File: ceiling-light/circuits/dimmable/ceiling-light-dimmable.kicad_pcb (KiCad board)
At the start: 2 copper layers, 100 x 100 mm, 21 parts, among them J1 Screw_Terminal_01x03, J2 Screw_Terminal_01x02, Q1 BT136-500, SW1 SW_Push, U1 LTV-817, U2 HLK-PM05, U3 MOC3021M, U4 WeMos_mini

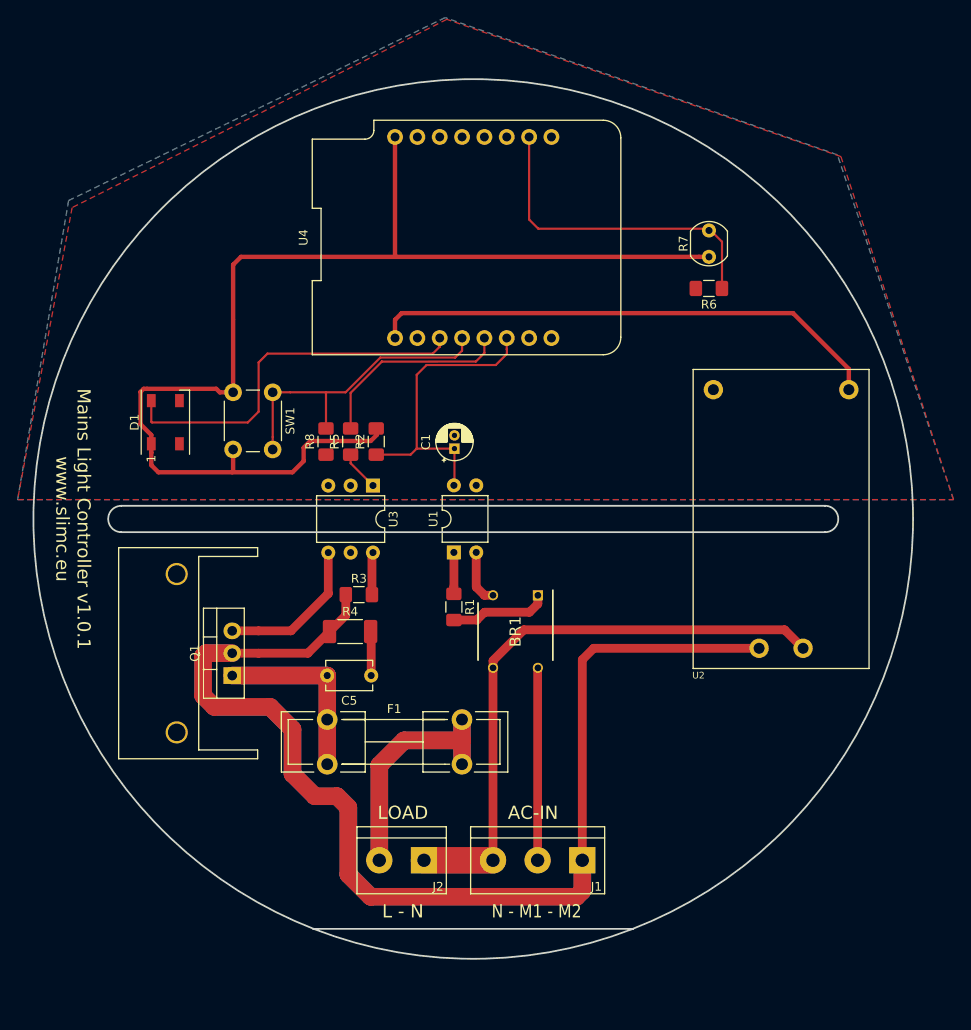
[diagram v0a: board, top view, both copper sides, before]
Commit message: work on dimmable circuit and git submodules
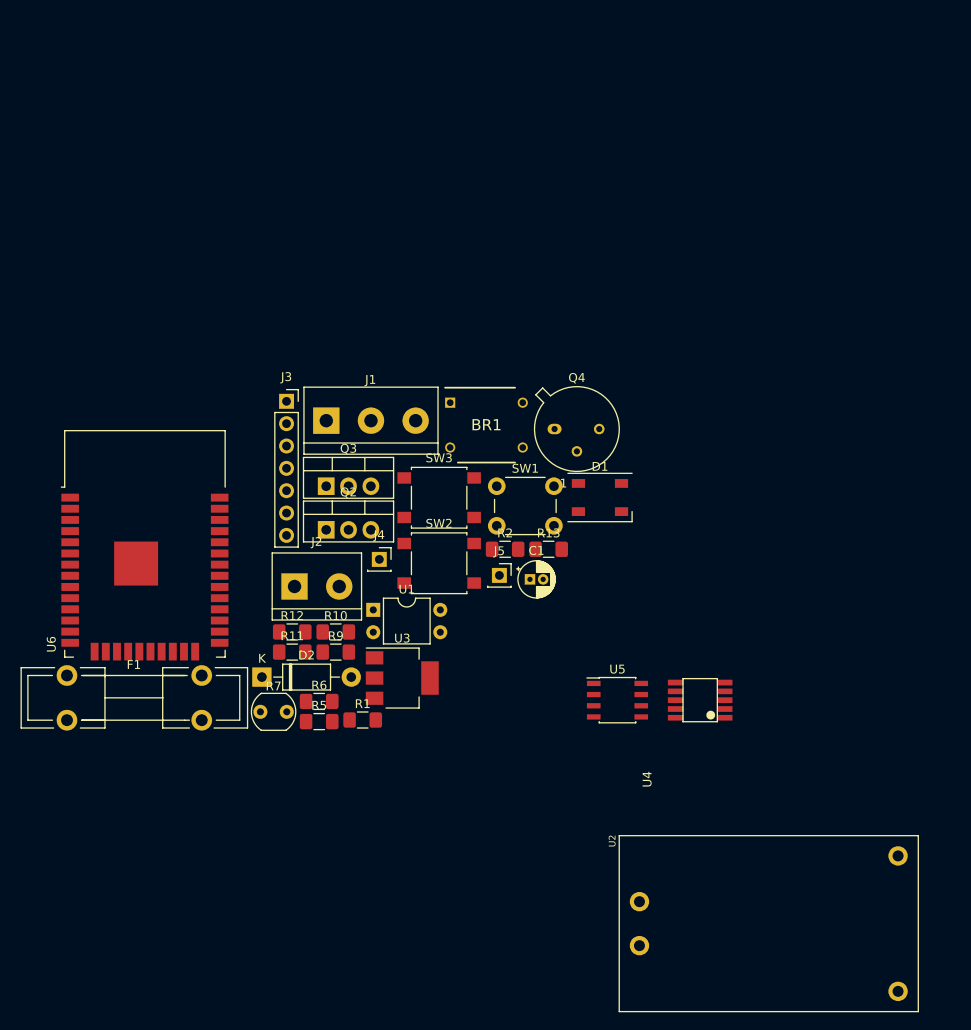
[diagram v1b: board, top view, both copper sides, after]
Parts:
- removed C5: 100NF, Capacitor_THT:C_Disc_D5.1mm_W3.2mm_P5.00mm
- removed Q1: BT136-500, slimc:TO-220-3_Vertical_Triode_Heatsink
- removed R3, R8: 10K, Resistor_SMD:R_1206_3216Metric_Pad1.42x1.75mm_HandSolder
- removed R4: 100R, Resistor_SMD:R_2010_5025Metric_Pad1.52x2.65mm_HandSolder
- added D2: 1N4007, Diode_THT:D_DO-41_SOD81_P10.16mm_Horizontal, F.Cu at (41.0, 83.0)
- added J3: Conn_01x07, Connector_PinSocket_2.54mm:PinSocket_1x07_P2.54mm_Vertical, F.Cu at (43.8, 51.6)
- added J4: Conn_01x01, Connector_PinSocket_2.54mm:PinSocket_1x01_P2.54mm_Vertical, F.Cu at (54.3, 69.6)
- added J5: Conn_01x01, Connector_PinSocket_2.54mm:PinSocket_1x01_P2.54mm_Vertical, F.Cu at (68.0, 71.4)
- added Q2: IRF840, Package_TO_SOT_THT:TO-220-3_Vertical, F.Cu at (48.3, 66.2)
- added Q3: IRF840, Package_TO_SOT_THT:TO-220-3_Vertical, F.Cu at (48.3, 61.3)
- added Q4: KSP44, Package_TO_SOT_THT:TO-39-3, F.Cu at (74.2, 54.8)
- added R10: 2M, Resistor_SMD:R_1206_3216Metric_Pad1.42x1.75mm_HandSolder, F.Cu at (49.4, 77.8)
- added R11: 1K, Resistor_SMD:R_1206_3216Metric_Pad1.42x1.75mm_HandSolder, F.Cu at (44.4, 80.1)
- added R12: 2M, Resistor_SMD:R_1206_3216Metric_Pad1.42x1.75mm_HandSolder, F.Cu at (44.4, 77.8)
- added R13: 2M, Resistor_SMD:R_1206_3216Metric_Pad1.42x1.75mm_HandSolder, F.Cu at (73.6, 68.4)
- added R9: 33K, Resistor_SMD:R_1206_3216Metric_Pad1.42x1.75mm_HandSolder, F.Cu at (49.4, 80.1)
- added SW2: SW_Push, Button_Switch_SMD:SW_SPST_B3S-1000, F.Cu at (61.1, 70.0)
- added SW3: SW_Push, Button_Switch_SMD:SW_SPST_B3S-1000, F.Cu at (61.1, 62.6)
- added U5: TMP36xS, Package_SO:SOIC-8_3.9x4.9mm_P1.27mm, F.Cu at (81.4, 85.6)
- added U6: ESP32-WROOM-32D, RF_Module:ESP32-WROOM-32, F.Cu at (27.7, 70.8)
- R5: value 33R -> 330K
- R6: value 10K -> 6K8
- U3: value MOC3021M -> AMS1117-3.3; footprint Package_DIP:DIP-6_W7.62mm -> Package_TO_SOT_SMD:SOT-223-3_TabPin2
- U4: value WeMos_mini -> FL51xxMX; footprint wemos-d1-mini:wemos-d1-mini-connectors-only -> slimc:FL51xxMX
- moved R7 72.6 mm to (40.8, 86.9), turned to 0 degrees
- moved R6 64.6 mm to (47.5, 85.7), turned to 0 degrees
- moved U4 58.6 mm to (90.8, 85.6), turned to 90 degrees
- moved J1 57.8 mm to (48.3, 53.8), turned to 0 degrees
- moved D1 50.1 mm to (79.4, 62.6), turned to 0 degrees
- moved U2 46.0 mm to (98.6, 111.0), turned to 0 degrees
- moved J2 34.4 mm to (44.7, 72.7), turned to 0 degrees
- moved R5 32.0 mm to (47.5, 88.0), turned to 0 degrees
- moved F1 30.0 mm to (18.8, 82.8)
- moved SW1 27.6 mm to (67.7, 61.3), turned to 0 degrees
- moved BR1 23.7 mm to (66.5, 54.3), turned to 0 degrees
- moved U3 22.1 mm to (56.9, 83.1), turned to 0 degrees
- moved R2 19.1 mm to (68.6, 68.4), turned to 0 degrees
- moved C1 17.2 mm to (71.4, 71.9), turned to 0 degrees
- moved R1 16.5 mm to (52.4, 87.9), turned to 0 degrees
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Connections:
- net M1_IN renamed /M1_IN
- net M2_IN renamed /M2_IN
- net N_MAIN renamed /N_MAIN
- C1 pad 1: D1 -> /MAINS_SENSE
- D1 pad 4: D4 -> /STATUS_LED
- F1 pad 1: L_OUT -> /L_OUT
- R2 pad 1: D1 -> /MAINS_SENSE
- R5 pad 1: Net-(R5-Pad1) -> Net-(Q4-Pad2)
- R5 pad 2: D2 -> Net-(D2-Pad1)
- R6 pad 1: A0 -> /LIGHT_SENSE
- R7 pad 2: A0 -> /LIGHT_SENSE
- SW1 pad 1: D3 -> Net-(SW1-Pad1)
- SW1 pad 2: +3V3 -> GND
- U1 pad 4: D1 -> /MAINS_SENSE
- U3 pad 1: Net-(R5-Pad1) -> GND
- U3 pad 2: GND -> +3V3
- U3 pad 3: Net-(U3-Pad3) -> +5V
- U4 pad 1: +5V -> Net-(R13-Pad2)
- U4 pad 10: A0 -> Net-(R10-Pad1)
- U4 pad 2: GND -> /DIMCN
- U4 pad 3: D4 -> +5V
- U4 pad 4: D3 -> /DIM_MODE
- U4 pad 5: D2 -> GND
- U4 pad 6: D1 -> Net-(C3-Pad1)
- U4 pad 7: RX -> Net-(Q4-Pad2)
- U4 pad 8: TX -> Net-(R12-Pad1)
- U4 pad 9: RST -> Net-(R11-Pad1)
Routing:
- net /M2_IN: track 204.0 -> 0.00 mm
- net +3V3: track 134.2 -> 0.00 mm
- net /N_MAIN: track 76.0 -> 0.00 mm
- net +5V: track 59.0 -> 0.00 mm
- net Net-(F1-Pad2): track 52.9 -> 0.00 mm
- net D4: track 43.1 -> 0.00 mm
- net L_OUT: track 41.8 -> 0.00 mm
- net A0: track 37.7 -> 0.00 mm
- net D3: track 35.6 -> 0.00 mm
- net D1: track 34.8 -> 0.00 mm
- net D2: track 22.8 -> 0.00 mm
- net /M1_IN: track 21.9 -> 0.00 mm
- net Net-(Q1-Pad3): track 17.4 -> 0.00 mm
- net Net-(BR1-Pad1): track 11.3 -> 0.00 mm
- net Net-(BR1-Pad2): track 6.24 -> 0.00 mm
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- removed copper zone on B.Cu, net GND
- removed copper zone on F.Cu, net GND
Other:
- board outline removed
- board text removed: "AC-IN"
- board text removed: "L - N"
- board text removed: "LOAD"
- board text removed: "Mains Light Controller v1.0.1 www.slimc.eu"
- board text removed: "N - M1 - M2"
